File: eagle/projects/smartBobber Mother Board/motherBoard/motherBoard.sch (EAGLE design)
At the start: 61 parts, among them J1 10118193-0001LF, J6 1053131202, Q1 2A/20V/150mΩ, Q2 MMBT3904, U1 MCP73831, U2 MT3608, U3 LTC3531ES6-3_3, Y1 ECS-40-S-4X

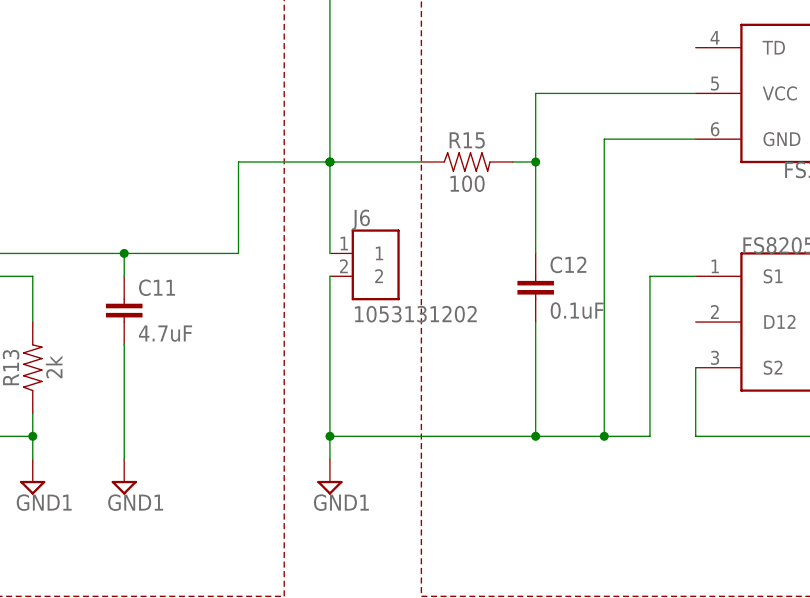
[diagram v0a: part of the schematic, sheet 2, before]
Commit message: I'm going through changes
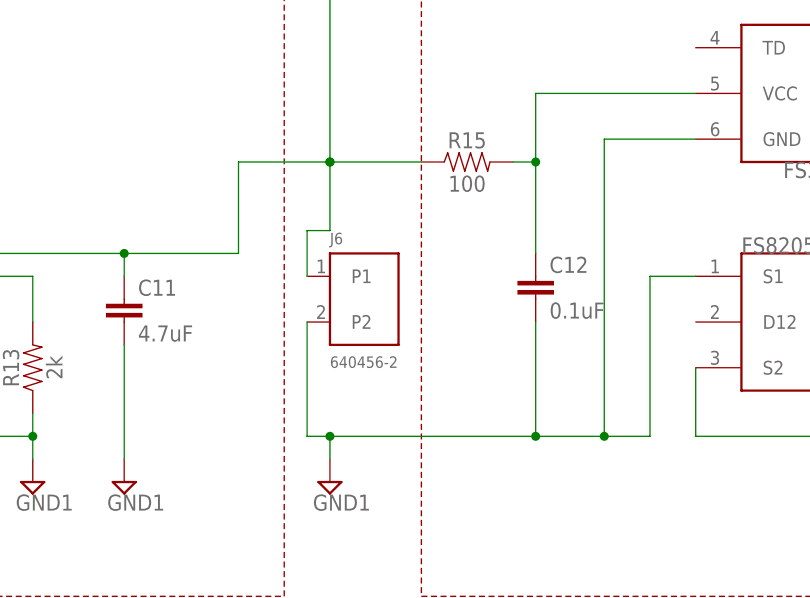
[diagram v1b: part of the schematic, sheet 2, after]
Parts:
- J6: value 1053131202 -> 640456-2; device 1053131202:1053131202 -> 640456-2:640456-2
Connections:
- net N$8: now also J6.P1; no longer J6.1
- net _12V: now also J6.P2; no longer J6.2
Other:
- moved on the sheet: J6
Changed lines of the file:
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@@
 <part name="SUPPLY14" library="supply2" library_urn="urn:adsk.eagle:library:372" deviceset="GND" device=""/>
 <part name="SUPPLY15" library="supply2" library_urn="urn:adsk.eagle:library:372" deviceset="GND" device=""/>
-<part name="J6" library="1053131202" deviceset="1053131202" device=""/>
 <part name="U$1" library="PIC16LF876A-I_SS" deviceset="PIC16LF876A-I/SS" device=""/>
 <part name="Y1" library="ECS-40-S-4X" deviceset="ECS-40-S-4X" device=""/>
@@
 <part name="U$6" library="SCMRCapacitor" deviceset="SCMR18G604SRBA0" device=""/>
 <part name="U$7" library="WNER50FET" deviceset="WNER50FET" device=""/>
+<part name="J6" library="640456-2" deviceset="640456-2" device=""/>
 </parts>
 <sheets>
@@
 <attribute name="VALUE" x="287.655" y="12.065" size="1.778" layer="96"/>
 </instance>
-<instance part="J6" gate="G$1" x="149.86" y="40.64" smashed="yes">
-<attribute name="NAME" x="147.312" y="43.6976" size="1.783609375" layer="95"/>
-<attribute name="VALUE" x="147.313540625" y="33.000609375" size="1.78251875" layer="96"/>
-</instance>
 <instance part="U1" gate="G$1" x="91.44" y="38.1" smashed="yes">
 <attribute name="NAME" x="83.82" y="43.688" size="1.778" layer="95"/>
@@
 <instance part="U$6" gate="G$1" x="320.04" y="88.9" smashed="yes"/>
 <instance part="U$7" gate="G$1" x="241.3" y="66.04" smashed="yes" rot="R90"/>
+<instance part="J6" gate="G$1" x="149.86" y="35.56" smashed="yes">
+<attribute name="NAME" x="144.77536875" y="41.661559375" size="1.271159375" layer="95"/>
+<attribute name="VALUE" x="144.772140625" y="27.928209375" size="1.271959375" layer="96"/>
+</instance>
 </instances>
 <busses>
@@
 <wire x1="144.78" y1="20.32" x2="167.64" y2="20.32" width="0.1524" layer="91"/>
 <pinref part="C12" gate="G$1" pin="2"/>
-<pinref part="J6" gate="G$1" pin="2"/>
 <wire x1="167.64" y1="33.02" x2="167.64" y2="20.32" width="0.1524" layer="91"/>
-<wire x1="144.78" y1="38.1" x2="144.78" y2="20.32" width="0.1524" layer="91"/>
-<junction x="144.78" y="20.32"/>
 <wire x1="167.64" y1="20.32" x2="175.26" y2="20.32" width="0.1524" layer="91"/>
 <junction x="167.64" y="20.32"/>
@@
 <wire x1="175.26" y1="53.34" x2="175.26" y2="20.32" width="0.1524" layer="91"/>
 <junction x="175.26" y="20.32"/>
+<pinref part="J6" gate="G$1" pin="P2"/>
+<wire x1="142.24" y1="33.02" x2="142.24" y2="20.32" width="0.1524" layer="91"/>
+<wire x1="142.24" y1="20.32" x2="144.78" y2="20.32" width="0.1524" layer="91"/>
+<junction x="144.78" y="20.32"/>
 </segment>
 <segment>
@@
 <wire x1="134.62" y1="50.8" x2="134.62" y2="40.64" width="0.1524" layer="91"/>
 <junction x="144.78" y="50.8"/>
-<pinref part="J6" gate="G$1" pin="1"/>
-<wire x1="144.78" y1="50.8" x2="144.78" y2="40.64" width="0.1524" layer="91"/>
 <wire x1="121.92" y1="40.64" x2="134.62" y2="40.64" width="0.1524" layer="91"/>
 <junction x="121.92" y="40.64"/>
-</segment>
-</net>
+<wire x1="144.78" y1="50.8" x2="144.78" y2="43.18" width="0.1524" layer="91"/>
+<wire x1="144.78" y1="43.18" x2="142.24" y2="43.18" width="0.1524" layer="91"/>
+<pinref part="J6" gate="G$1" pin="P1"/>
+<wire x1="142.24" y1="43.18" x2="142.24" y2="38.1" width="0.1524" layer="91"/>
+</segment>
+</net>
